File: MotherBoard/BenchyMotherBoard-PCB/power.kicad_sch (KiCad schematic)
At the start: 449 parts, among them J1 PWR CONN, J26 PWR CONN, J3 EN1 JUMPER, J4 EN1 JUMPER, Q1 MMBT2222A, Q2 MMBT2222A, Q3 MMBT2222A, Q4 MMBT2222A, U1 AM6254ATCGGAALW, U10 AP3401, U11 INA231AIYFFR, U12 AP2127K-1.2, U14 INA231AIYFFR, U15 MAX15027, U16 INA231AIYFFR, U17 TLV7103318, U18 USB7206C, U19 AP2127K-1.2, U2 MAX16043, U20 INA231AIYFFR, U21 TLV75518PDRV, U22 TPS54308, U23 KSZ9021RN, U24 KSZ9021RN, U3 TPS65400RGZT, U4 PCA9517, U5 SiI9022ACNU, U6 TLV759P, U7 MAX809, U8 INA231AIYFFR

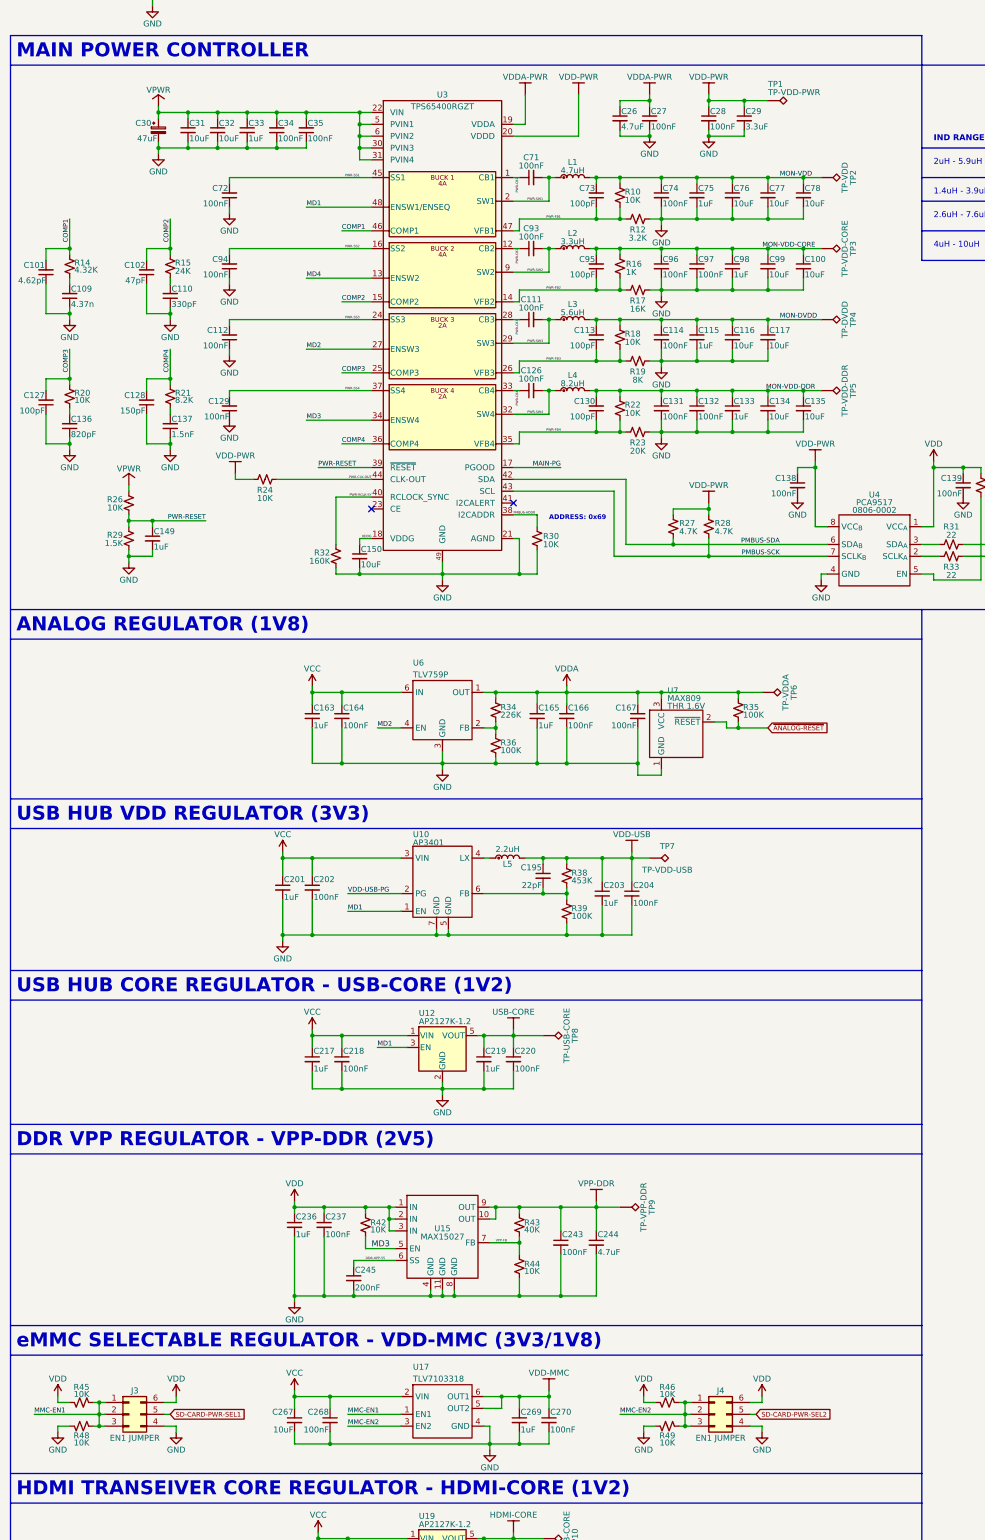
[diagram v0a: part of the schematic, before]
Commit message: (WIP) Still laying out PCB
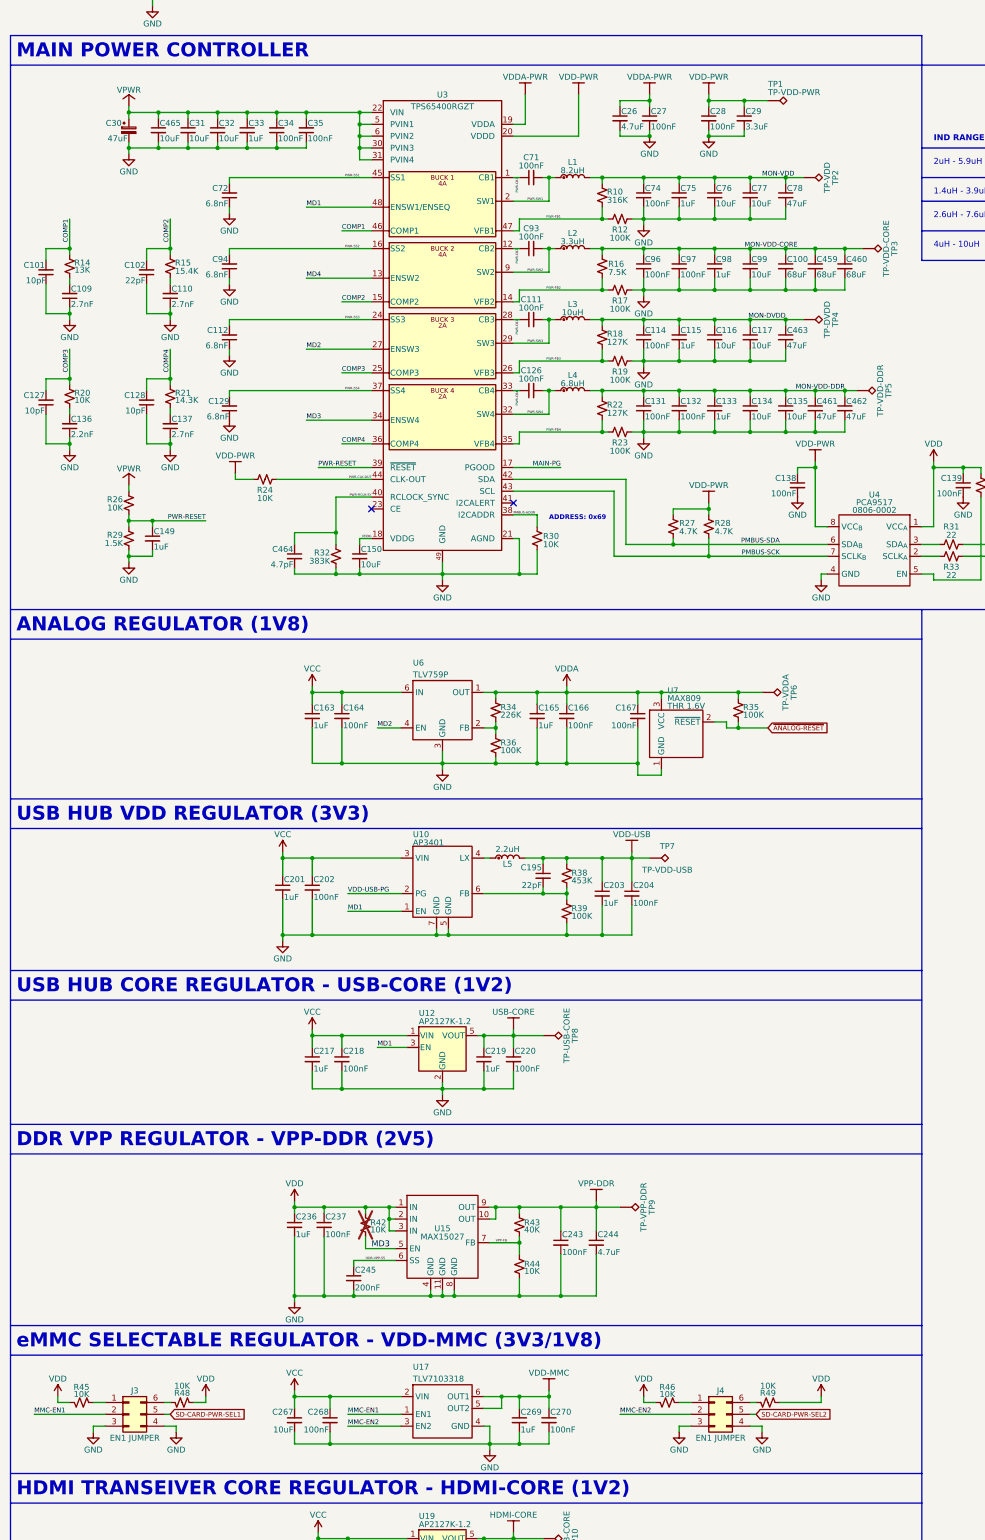
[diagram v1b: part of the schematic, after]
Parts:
- removed C113, C130, C73, C95: 100pF, Capacitor_SMD:C_0402_1005Metric, symbol Daxxn_Device:C
- added C459, C460: 68uF, Capacitor_SMD:C_1206_3216Metric, symbol Daxxn_Device:C
- added C461, C462, C463: 47uF, Capacitor_SMD:C_1206_3216Metric, symbol Daxxn_Device:C
- added C464: 4.7pF, Capacitor_SMD:C_0402_1005Metric, symbol Daxxn_Device:C
- added C465: 10uF, Capacitor_SMD:C_1210_3225Metric, symbol Daxxn_Device:C
- C100: value 10uF -> 68uF; footprint Capacitor_SMD:C_1210_3225Metric -> Capacitor_SMD:C_1206_3216Metric
- C101: value 4.62pF -> 10pF
- C102: value 47pF -> 22pF
- C109: value 4.37n -> 2.7nF
- C110: value 330pF -> 2.7nF
- C112, C129, C72, C94: value 100nF -> 6.8nF
- C127: value 100pF -> 10pF
- C128: value 150pF -> 10pF
- C136: value 820pF -> 2.2nF
- C137: value 1.5nF -> 2.7nF
- C78: value 10uF -> 47uF; footprint Capacitor_SMD:C_1210_3225Metric -> Capacitor_SMD:C_1206_3216Metric
- L1: value 4.7uH -> 8.2uH
- L3: value 5.6uH -> 10uH
- L4: value 8.2uH -> 6.8uH
- R10: value 10K -> 316K
- R12: value 3.2K -> 100K
- R14: value 4.32K -> 13K
- R15: value 24K -> 15.4K
- R16: value 1K -> 7.5K
- R17: value 16K -> 100K
- R18, R22: value 10K -> 127K
- R19: value 8K -> 100K
- R21: value 8.2K -> 14.3K
- R23: value 20K -> 100K
- R32: value 160K -> 383K
- R42: now not fitted
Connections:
- net GND: now also J3.3 (Pin_3), J4.3 (Pin_3), C459.2, C460.2, C461.2, C462.2, C463.2, C464.2, C465.2; no longer R48.1, R49.1
- net MMC-EN1: no longer J3.1 (Pin_1), J3.3 (Pin_3), R45.1, R48.2
- net MMC-EN2: no longer J4.1 (Pin_1), J4.3 (Pin_3), R46.1, R49.2
- net MON-DVDD: now also C463.1
- net MON-VDD-CORE: now also C459.1, C460.1
- net MON-VDD-DDR: now also C461.1, C462.1
- net PWR-RCLK-SY: now also C464.1
- net VDD: now also R48.1, R49.1; no longer J3.6 (Pin_6), J4.6 (Pin_6)
- net VPWR: now also C465.1
- new net: J3.1 (Pin_1), R45.1
- new net: J3.6 (Pin_6), R48.2
- new net: J4.1 (Pin_1), R46.1
- new net: J4.6 (Pin_6), R49.2
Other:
- moved on the sheet: C100, C114, C115, C116, C117, C131, C132, C133, C134, C135, C30, C74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
